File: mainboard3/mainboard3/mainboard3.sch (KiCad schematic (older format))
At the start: 31 parts, among them J0 Conn_01x18, J1 Conn_01x18, J2 Conn_01x18, J4 Conn_01x18, J5 Conn_01x18, T0 Screw_Terminal_01x06, T1 Screw_Terminal_01x06, T10 Screw_Terminal_01x06, T11 Screw_Terminal_01x06, T12 Screw_Terminal_01x06, T2 Screw_Terminal_01x06, T3 Screw_Terminal_01x06, T4 Screw_Terminal_01x06, T5 Screw_Terminal_01x06, T6 Screw_Terminal_01x06, T7 Screw_Terminal_01x06, T8 Screw_Terminal_01x06, T9 Screw_Terminal_01x06, U1 STM32_F4xx, U2 ModuleINA3221, U3 ModuleINA3221, U4 ModuleINA3221, U5 ModuleINA3221, U6 ULN2803A, U7 ULN2803A, X1 Screw_Terminal_01x04

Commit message: mainboard3 again
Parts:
- removed T0, T1, T12, T2, T3, T4: Screw_Terminal_01x06, Connector_PinHeader_2.54mm:PinHeader_1x06_P2.54mm_Vertical, symbol Connector:Screw_Terminal_01x06
- added 10k1, R1, R20, R21, R22, R23, R24, R25, R26, R27: R, Resistor_THT:R_Axial_DIN0207_L6.3mm_D2.5mm_P7.62mm_Horizontal, symbol Device:R
- added C1, C2, C3, C4, C5: 100nF, Capacitor_THT:C_Disc_D3.4mm_W2.1mm_P2.50mm, symbol Device:C
- added C6: 0.1µF, Capacitor_THT:C_Disc_D3.4mm_W2.1mm_P2.50mm, symbol Device:CP
- added C7: 10µF, Capacitor_THT:CP_Radial_Tantal_D5.0mm_P2.50mm, symbol Device:CP
- added J7: Conn_01x02_Female, Connector_PinHeader_2.54mm:PinHeader_1x02_P2.54mm_Vertical, symbol Connector:Conn_01x02_Female
- added JG2, JG3, JG4, JG5: Conn_01x03_Female, Connector_PinHeader_2.54mm:PinHeader_1x03_P2.54mm_Vertical, symbol Connector:Conn_01x03_Female
- added JI2, JI3, JI4, JI5: Conn_01x06_Female, Connector_PinHeader_2.54mm:PinHeader_1x06_P2.54mm_Vertical, symbol Connector:Conn_01x06_Female
- added JLED1, JLED2: Conn_01x08_Female, Connector_PinHeader_2.54mm:PinHeader_1x08_P2.54mm_Vertical, symbol Connector:Conn_01x08_Female
- added JT_0_1, JT_0_2, JT_0_3, JT_1_1, JT_1_2, JT_1_3, JT_2_1, JT_2_2, JT_3_1, JT_3_2, JT_4_1, JT_5_1: Screw_Terminal_01x02, Connector_PinHeader_2.54mm:PinHeader_1x02_P2.54mm_Vertical, symbol Connector:Screw_Terminal_01x02
- added R10, R11, R12, R13, R14, R15, R16, R17, R18, R19, R3, R4, R5, R6, R7, R8, R9: 10k, Resistor_THT:R_Axial_DIN0207_L6.3mm_D2.5mm_P7.62mm_Horizontal, symbol Device:R
- added R28: 510, Resistor_THT:R_Axial_DIN0207_L6.3mm_D2.5mm_P7.62mm_Horizontal, symbol Device:R
- added R29: 200, Resistor_THT:R_Axial_DIN0207_L6.3mm_D2.5mm_P7.62mm_Horizontal, symbol Device:R
- added R30: 240, Resistor_THT:R_Axial_DIN0207_L6.3mm_D2.5mm_P7.62mm_Horizontal, symbol Device:R
- added SW1: SW_DIP_x01, Connector_PinHeader_2.54mm:PinHeader_1x02_P2.54mm_Vertical, symbol Switch:SW_DIP_x01
- added U10: LM317_TO220, Package_TO_SOT_THT:TO-220-3_Vertical, symbol Regulator_Linear:LM317_TO-220
- added U9: ULN2803A, Package_DIP:DIP-18_W7.62mm, symbol Transistor_Array:ULN2803A
- gave numbers to parts that had none: 4
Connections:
- net labels added: BOARD_LED, BOARD_LED2, CAN_RX, CAN_TX, I10A, I10B, I11A, I11B, I12A, I12B, I1A, I1B, I2A, I2B, I3A, I3B, I4A, I4B, I5A, I5B, I6A, I6B, I7A, I7B, I8A, I8B, I9A, I9B, LED3, LED4, LED5, LED6, LED7, LED8, V5
- wire segments 232 -> 353
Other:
- moved on the sheet: U3, U4, U5

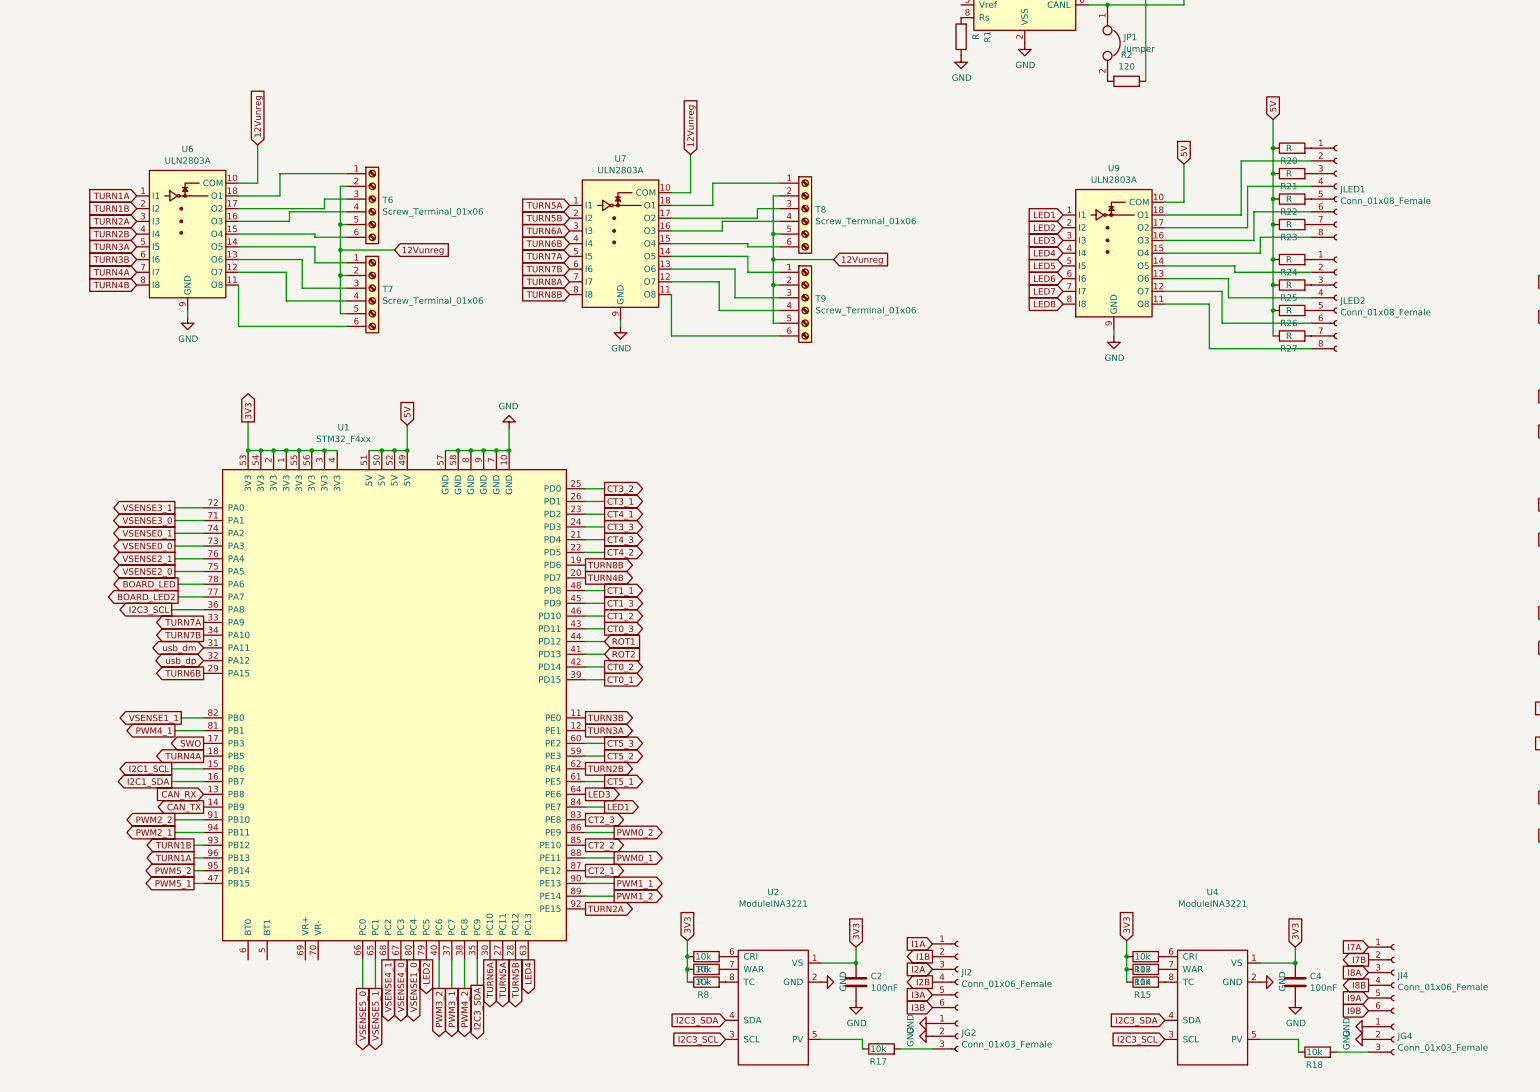
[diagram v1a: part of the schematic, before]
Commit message: mainboard3  routing
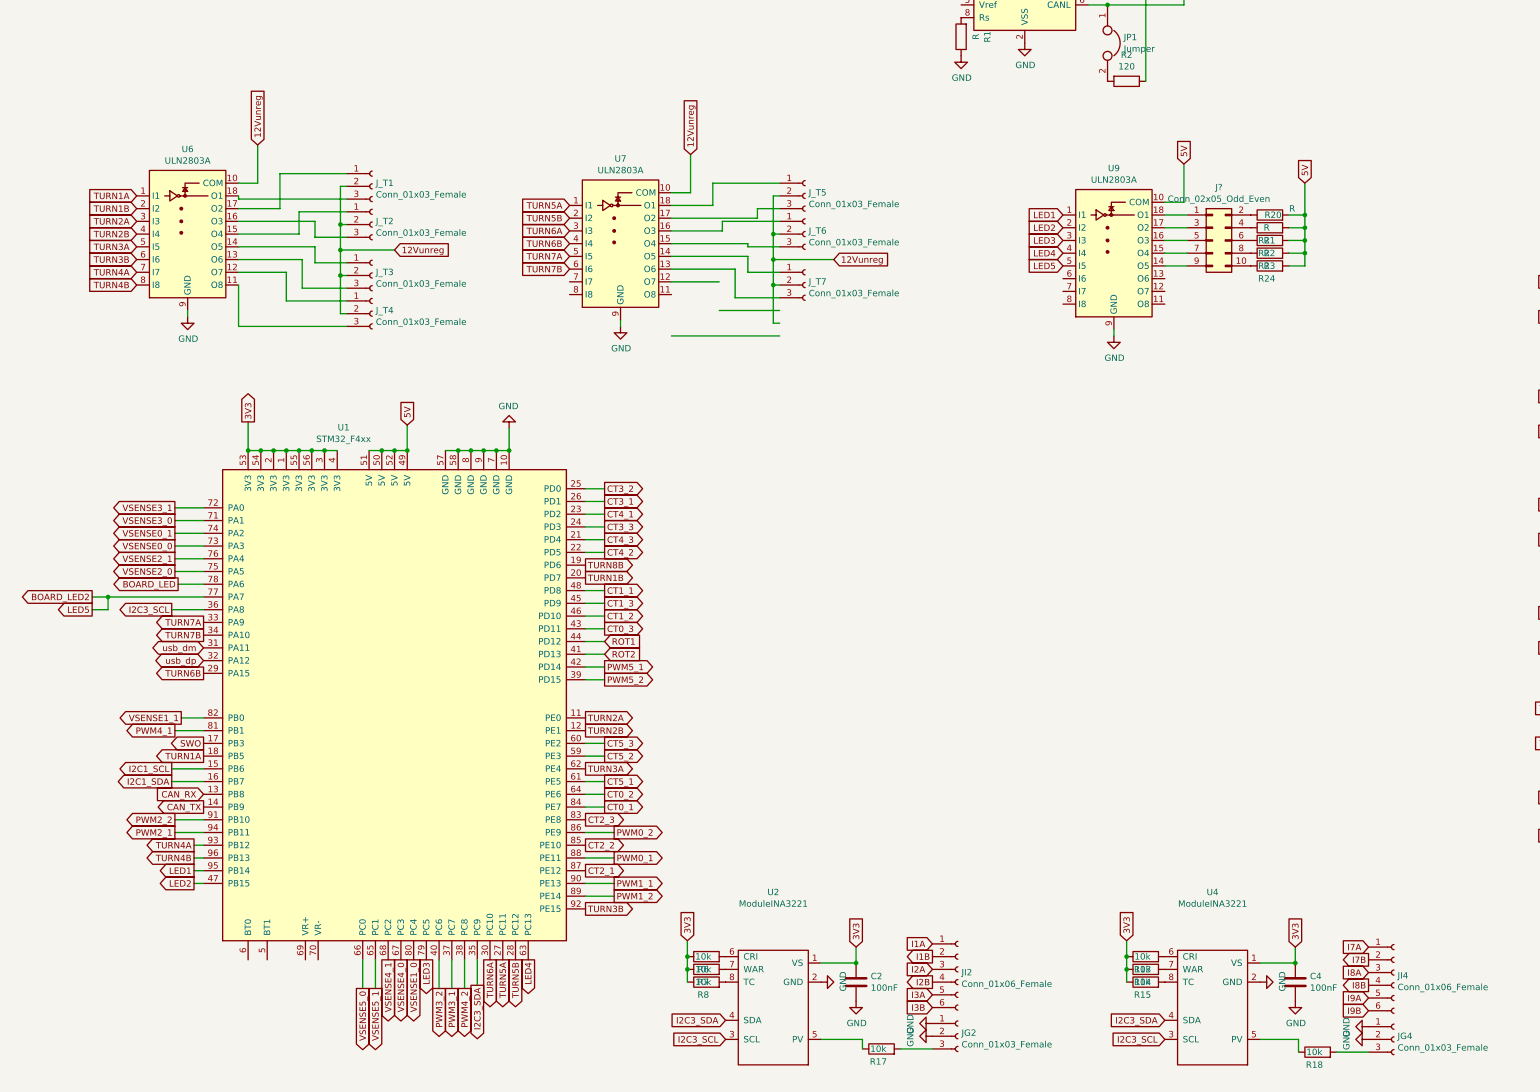
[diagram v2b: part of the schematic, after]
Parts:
- removed JLED1, JLED2: Conn_01x08_Female, Connector_PinHeader_2.54mm:PinHeader_1x08_P2.54mm_Vertical, symbol Connector:Conn_01x08_Female
- removed R25, R26, R27: R, Resistor_THT:R_Axial_DIN0207_L6.3mm_D2.5mm_P7.62mm_Horizontal, symbol Device:R
- removed T6, T7, T8, T9: Screw_Terminal_01x06, Connector_PinHeader_2.54mm:PinHeader_1x06_P2.54mm_Vertical, symbol Connector:Screw_Terminal_01x06
- added J?: Conn_02x05_Odd_Even, symbol Connector_Generic:Conn_02x05_Odd_Even
- added J_T1, J_T2, J_T3, J_T4, J_T5, J_T6, J_T7: Conn_01x03_Female, Connector_PinHeader_2.54mm:PinHeader_1x03_P2.54mm_Vertical, symbol Connector:Conn_01x03_Female
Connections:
- net labels removed: LED6, LED7, LED8, TURN8A
- wire segments 353 -> 337
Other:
- moved on the sheet: R20, R21, R22, R23, R24

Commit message: before moving to kicad6
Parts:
- removed J6: Conn_01x06_Female, Connector_PinHeader_2.54mm:PinHeader_1x06_P2.54mm_Vertical, symbol Connector:Conn_01x06_Female
- added C8: 0.1µF, Capacitor_THT:C_Disc_D3.4mm_W2.1mm_P2.50mm, symbol Device:CP
- added C9: 10µF, Capacitor_THT:CP_Radial_Tantal_D5.0mm_P2.50mm, symbol Device:CP
- added J_BUS1, J_GUI1: Conn_01x05_Female, Connector_PinHeader_2.54mm:PinHeader_1x05_P2.54mm_Vertical, symbol Connector:Conn_01x05_Female
- added R25, R26: R, Resistor_THT:R_Axial_DIN0207_L6.3mm_D2.5mm_P7.62mm_Horizontal, symbol Device:R
- added R27: 240, Resistor_THT:R_Axial_DIN0207_L6.3mm_D2.5mm_P7.62mm_Horizontal, symbol Device:R
- added SW2, SW3: SW_DIP_x01, Connector_PinHeader_2.54mm:PinHeader_1x02_P2.54mm_Vertical, symbol Switch:SW_DIP_x01
- added U11: LM317_TO220, Package_TO_SOT_THT:TO-220-3_Vertical, symbol Regulator_Linear:LM317_TO-220
- J8: renamed from J?; footprint (none) -> Connector_PinHeader_2.54mm:PinHeader_2x05_P2.54mm_Vertical
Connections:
- net labels added: 12V
- net labels removed: +12V, +5V, TRIG, TT2_1, V5
- wire segments 337 -> 365
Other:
- moved on the sheet: C6, C7, J7, R28, R29, R30, SW1, U10
